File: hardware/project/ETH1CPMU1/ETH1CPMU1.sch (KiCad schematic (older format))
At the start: 0 parts

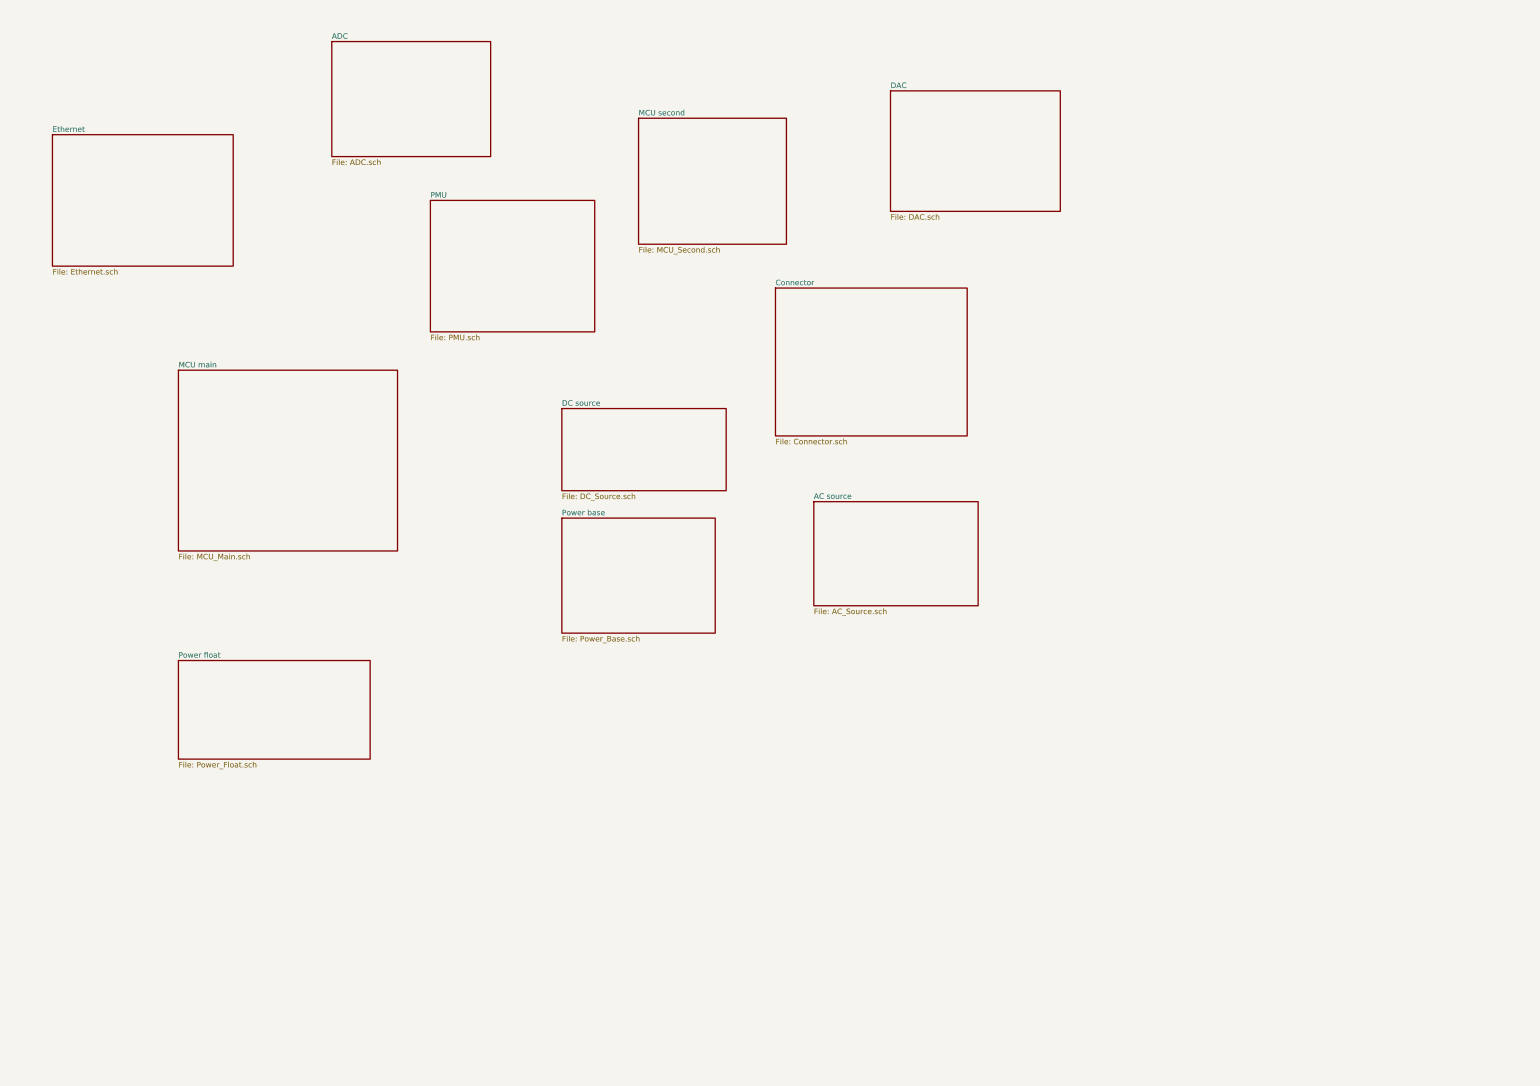
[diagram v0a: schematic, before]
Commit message: Schematic design
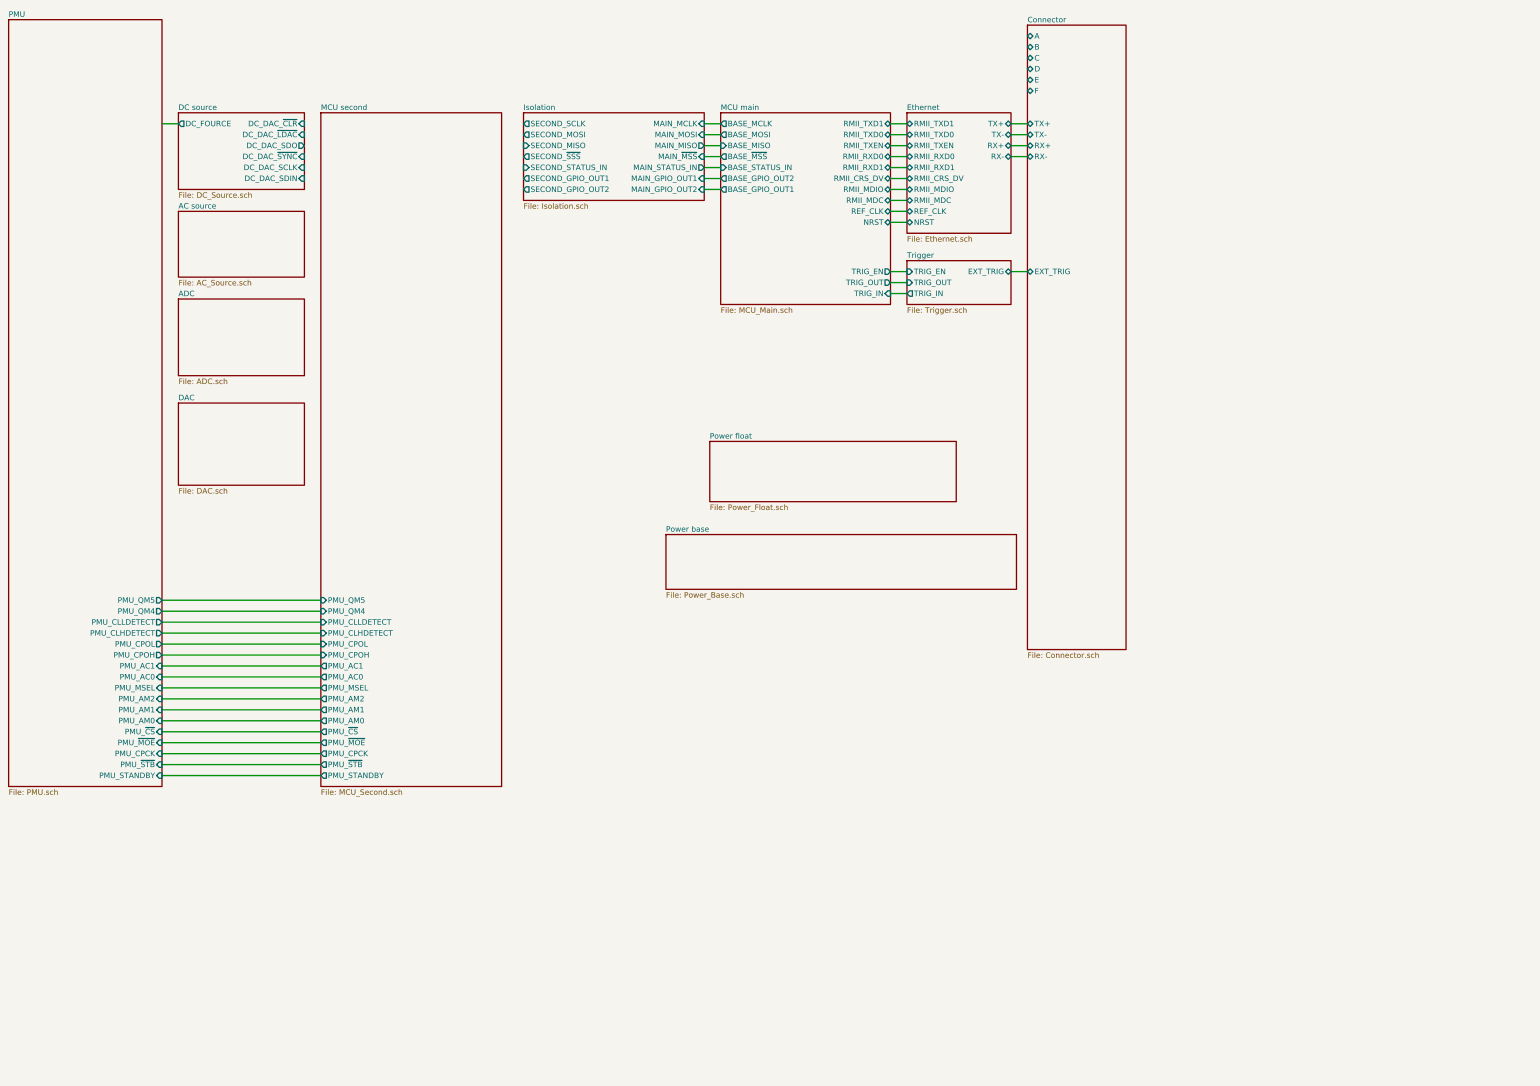
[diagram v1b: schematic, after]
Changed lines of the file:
@@
 $Descr A4 11693 8268
 encoding utf-8
-Sheet 1 12
+Sheet 1 14
 Title ""
 Date ""
@@
 $EndDescr
 $Sheet
-S 7900 3050 1750 1350
+S 10200 650  900  5700
 U 5DCED2F4
 F0 "Connector" 50
 F1 "Connector.sch" 50
-$EndSheet
-$Sheet
-S 2450 3800 2000 1650
+F2 "RX+" B L 10200 1750 50
+F3 "TX+" B L 10200 1550 50
+F4 "RX-" B L 10200 1850 50
+F5 "TX-" B L 10200 1650 50
+F6 "EXT_TRIG" B L 10200 2900 50
+F7 "A" B L 10200 750 50
+F8 "B" B L 10200 850 50
+F9 "C" B L 10200 950 50
+F10 "D" B L 10200 1050 50
+F11 "E" B L 10200 1150 50
+F12 "F" B L 10200 1250 50
+$EndSheet
+$Sheet
+S 7400 1450 1550 1750
 U 5DCED281
 F0 "MCU main" 50
 F1 "MCU_Main.sch" 50
-$EndSheet
-$Sheet
-S 1300 1650 1650 1200
+F2 "RMII_TXD1" B R 8950 1550 50
+F3 "RMII_TXD0" B R 8950 1650 50
+F4 "RMII_TXEN" B R 8950 1750 50
+F5 "RMII_RXD0" B R 8950 1850 50
+F6 "RMII_RXD1" B R 8950 1950 50
+F7 "RMII_CRS_DV" B R 8950 2050 50
+F8 "RMII_MDIO" B R 8950 2150 50
+F9 "RMII_MDC" B R 8950 2250 50
+F10 "REF_CLK" B R 8950 2350 50
+F11 "NRST" B R 8950 2450 50
+F12 "BASE_MCLK" O L 7400 1550 50
+F13 "BASE_MOSI" O L 7400 1650 50
+F14 "BASE_MISO" I L 7400 1750 50
+F15 "BASE_~MSS" O L 7400 1850 50
+F16 "TRIG_EN" O R 8950 2900 50
+F17 "TRIG_OUT" O R 8950 3000 50
+F18 "TRIG_IN" I R 8950 3100 50
+F19 "BASE_STATUS_IN" I L 7400 1950 50
+F20 "BASE_GPIO_OUT2" O L 7400 2050 50
+F21 "BASE_GPIO_OUT1" O L 7400 2150 50
+$EndSheet
+$Sheet
+S 9100 1450 950  1100
 U 5DD0AEA4
 F0 "Ethernet" 50
 F1 "Ethernet.sch" 50
-$EndSheet
-$Sheet
-S 5950 5150 1400 1050
+F2 "TX+" B R 10050 1550 50
+F3 "TX-" B R 10050 1650 50
+F4 "RX+" B R 10050 1750 50
+F5 "RX-" B R 10050 1850 50
+F6 "RMII_TXD1" B L 9100 1550 50
+F7 "RMII_TXD0" B L 9100 1650 50
+F8 "RMII_TXEN" B L 9100 1750 50
+F9 "RMII_RXD0" B L 9100 1850 50
+F10 "RMII_RXD1" B L 9100 1950 50
+F11 "RMII_CRS_DV" B L 9100 2050 50
+F12 "RMII_MDIO" B L 9100 2150 50
+F13 "RMII_MDC" B L 9100 2250 50
+F14 "NRST" B L 9100 2450 50
+F15 "REF_CLK" B L 9100 2350 50
+$EndSheet
+$Sheet
+S 6900 5300 3200 500
 U 5DD0B0B8
 F0 "Power base" 50
@@
 $EndSheet
 $Sheet
-S 2450 6450 1750 900
+S 7300 4450 2250 550
 U 5DD0DBE6
 F0 "Power float" 50
@@
 $EndSheet
 $Sheet
-S 6650 1500 1350 1150
+S 3750 1450 1650 6150
 U 5DF35BC8
 F0 "MCU second" 50
 F1 "MCU_Second.sch" 50
-$EndSheet
-$Sheet
-S 4750 2250 1500 1200
+F2 "PMU_STANDBY" O L 3750 7500 50
+F3 "PMU_~STB" O L 3750 7400 50
+F4 "PMU_CPCK" O L 3750 7300 50
+F5 "PMU_~MOE" O L 3750 7200 50
+F6 "PMU_~CS" O L 3750 7100 50
+F7 "PMU_AM0" O L 3750 7000 50
+F8 "PMU_AM1" O L 3750 6900 50
+F9 "PMU_AM2" O L 3750 6800 50
+F10 "PMU_MSEL" O L 3750 6700 50
+F11 "PMU_AC0" O L 3750 6600 50
+F12 "PMU_AC1" O L 3750 6500 50
+F13 "PMU_CPOH" I L 3750 6400 50
+F14 "PMU_CPOL" I L 3750 6300 50
+F15 "PMU_CLHDETECT" I L 3750 6200 50
+F16 "PMU_CLLDETECT" I L 3750 6100 50
+F17 "PMU_QM4" I L 3750 6000 50
+F18 "PMU_QM5" I L 3750 5900 50
+$EndSheet
+$Sheet
+S 2450 1450 1150 700
+U 5DF36C0B
+F0 "DC source" 50
+F1 "DC_Source.sch" 50
+F2 "DC_FOURCE" O L 2450 1550 50
+F3 "DC_DAC_~CLR" I R 3600 1550 50
+F4 "DC_DAC_~LDAC" I R 3600 1650 50
+F5 "DC_DAC_SDO" O R 3600 1750 50
+F6 "DC_DAC_~SYNC" I R 3600 1850 50
+F7 "DC_DAC_SCLK" I R 3600 1950 50
+F8 "DC_DAC_SDIN" I R 3600 2050 50
+$EndSheet
+$Sheet
+S 2450 2350 1150 600
+U 5DF36C25
+F0 "AC source" 50
+F1 "AC_Source.sch" 50
+$EndSheet
+$Sheet
+S 2450 3150 1150 700
+U 5DF36C38
+F0 "ADC" 50
+F1 "ADC.sch" 50
+$EndSheet
+$Sheet
+S 2450 4100 1150 750
+U 5DF36C70
+F0 "DAC" 50
+F1 "DAC.sch" 50
+$EndSheet
+Wire Wire Line
+	9100 2450 8950 2450
+Wire Wire Line
+	8950 2350 9100 2350
+Wire Wire Line
+	9100 2250 8950 2250
+Wire Wire Line
+	8950 2150 9100 2150
+Wire Wire Line
+	9100 2050 8950 2050
+Wire Wire Line
+	8950 1950 9100 1950
+Wire Wire Line
+	9100 1850 8950 1850
+Wire Wire Line
+	8950 1750 9100 1750
+Wire Wire Line
+	8950 1650 9100 1650
+Wire Wire Line
+	9100 1550 8950 1550
+$Sheet
+S 9100 2800 950  400
+U 5DD52C08
+F0 "Trigger" 50
+F1 "Trigger.sch" 50
+F2 "EXT_TRIG" B R 10050 2900 50
+F3 "TRIG_EN" I L 9100 2900 50
+F4 "TRIG_OUT" I L 9100 3000 50
+F5 "TRIG_IN" O L 9100 3100 50
+$EndSheet
+Wire Wire Line
+	9100 2900 8950 2900
+Wire Wire Line
+	8950 3000 9100 3000
+Wire Wire Line
+	9100 3100 8950 3100
+Wire Wire Line
+	10200 2900 10050 2900
+Wire Wire Line
+	10200 1850 10050 1850
+Wire Wire Line
+	10050 1750 10200 1750
+Wire Wire Line
+	10200 1650 10050 1650
+Wire Wire Line
+	10200 1550 10050 1550
+$Sheet
+S 5600 1450 1650 800
+U 5DD672F1
+F0 "Isolation" 50
+F1 "Isolation.sch" 50
+F2 "MAIN_GPIO_OUT1" I R 7250 2050 50
+F3 "MAIN_~MSS" I R 7250 1850 50
+F4 "MAIN_MISO" O R 7250 1750 50
+F5 "MAIN_MOSI" I R 7250 1650 50
+F6 "MAIN_MCLK" I R 7250 1550 50
+F7 "MAIN_STATUS_IN" O R 7250 1950 50
+F8 "MAIN_GPIO_OUT2" I R 7250 2150 50
+F9 "SECOND_~SSS" O L 5600 1850 50
+F10 "SECOND_MISO" I L 5600 1750 50
+F11 "SECOND_MOSI" O L 5600 1650 50
+F12 "SECOND_SCLK" O L 5600 1550 50
+F13 "SECOND_GPIO_OUT1" O L 5600 2050 50
+F14 "SECOND_STATUS_IN" I L 5600 1950 50
+F15 "SECOND_GPIO_OUT2" O L 5600 2150 50
+$EndSheet
+$Sheet
+S 900  600  1400 7000
 U 5DF36410
 F0 "PMU" 50
 F1 "PMU.sch" 50
-$EndSheet
-$Sheet
-S 5950 4150 1500 750
-U 5DF36C0B
-F0 "DC source" 50
-F1 "DC_Source.sch" 50
-$EndSheet
-$Sheet
-S 8250 5000 1500 950
-U 5DF36C25
-F0 "AC source" 50
-F1 "AC_Source.sch" 50
-$EndSheet
-$Sheet
-S 3850 800  1450 1050
-U 5DF36C38
-F0 "ADC" 50
-F1 "ADC.sch" 50
-$EndSheet
-$Sheet
-S 8950 1250 1550 1100
-U 5DF36C70
-F0 "DAC" 50
-F1 "DAC.sch" 50
-$EndSheet
+F2 "PMU_STANDBY" I R 2300 7500 50
+F3 "PMU_~STB" I R 2300 7400 50
+F4 "PMU_CPCK" I R 2300 7300 50
+F5 "PMU_~MOE" I R 2300 7200 50
+F6 "PMU_~CS" I R 2300 7100 50
+F7 "PMU_AM0" I R 2300 7000 50
+F8 "PMU_AM1" I R 2300 6900 50
+F9 "PMU_AM2" I R 2300 6800 50
+F10 "PMU_MSEL" I R 2300 6700 50
+F11 "PMU_AC0" I R 2300 6600 50
+F12 "PMU_AC1" I R 2300 6500 50
+F13 "PMU_CPOH" O R 2300 6400 50
+F14 "PMU_CPOL" O R 2300 6300 50
+F15 "PMU_CLHDETECT" O R 2300 6200 50
+F16 "PMU_CLLDETECT" O R 2300 6100 50
+F17 "PMU_QM4" O R 2300 6000 50
+F18 "PMU_QM5" O R 2300 5900 50
+$EndSheet
+Wire Wire Line
+	2300 7500 3750 7500
+Wire Wire Line
+	3750 7400 2300 7400
+Wire Wire Line
+	2300 7300 3750 7300
+Wire Wire Line
+	3750 7200 2300 7200
+Wire Wire Line
+	2300 7100 3750 7100
+Wire Wire Line
+	3750 7000 2300 7000
+Wire Wire Line
+	2300 6900 3750 6900
+Wire Wire Line
+	2300 6800 3750 6800
+Wire Wire Line
+	2300 6700 3750 6700
+Wire Wire Line
+	3750 6600 2300 6600
+Wire Wire Line
+	2300 6500 3750 6500
+Wire Wire Line
+	3750 6400 2300 6400
+Wire Wire Line
+	2300 6300 3750 6300
+Wire Wire Line
+	3750 6200 2300 6200
+Wire Wire Line
+	2300 6100 3750 6100
+Wire Wire Line
+	3750 6000 2300 6000
+Wire Wire Line
+	2300 5900 3750 5900
+Wire Wire Line
+	2450 1550 2300 1550
+Wire Wire Line
+	7400 1550 7250 1550
+Wire Wire Line
+	7250 1650 7400 1650
+Wire Wire Line
+	7400 1750 7250 1750
+Wire Wire Line
+	7250 1850 7400 1850
+Wire Wire Line
+	7400 1950 7250 1950
+Wire Wire Line
+	7250 2050 7400 2050
+Wire Wire Line
+	7400 2150 7250 2150
 $EndSCHEMATC

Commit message: Schematic design
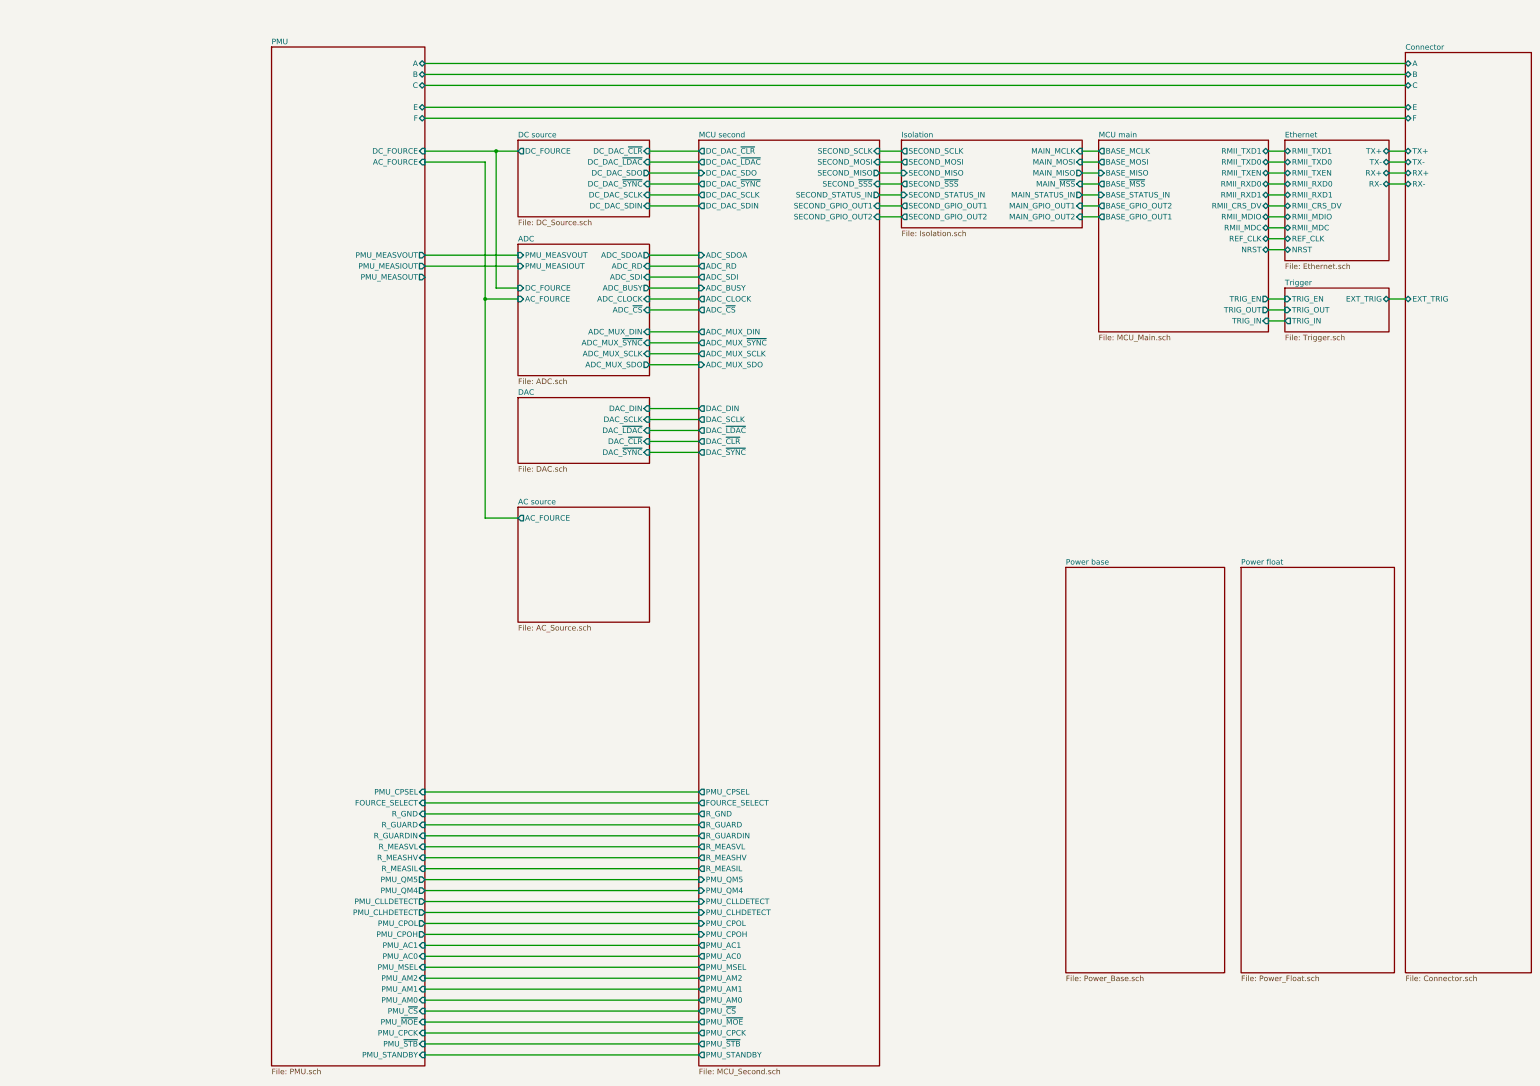
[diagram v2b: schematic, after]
